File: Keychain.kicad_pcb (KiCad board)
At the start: 4 copper layers, 106.7 x 78.7 mm, 57 parts, among them J1 Micro_SD_Card, J2 Conn_01x04, U1 IMX6UL_BGA289, U2 DDR3_BGA96, U3 AZ1117C-3.3, U4 AZ1117C-1.5

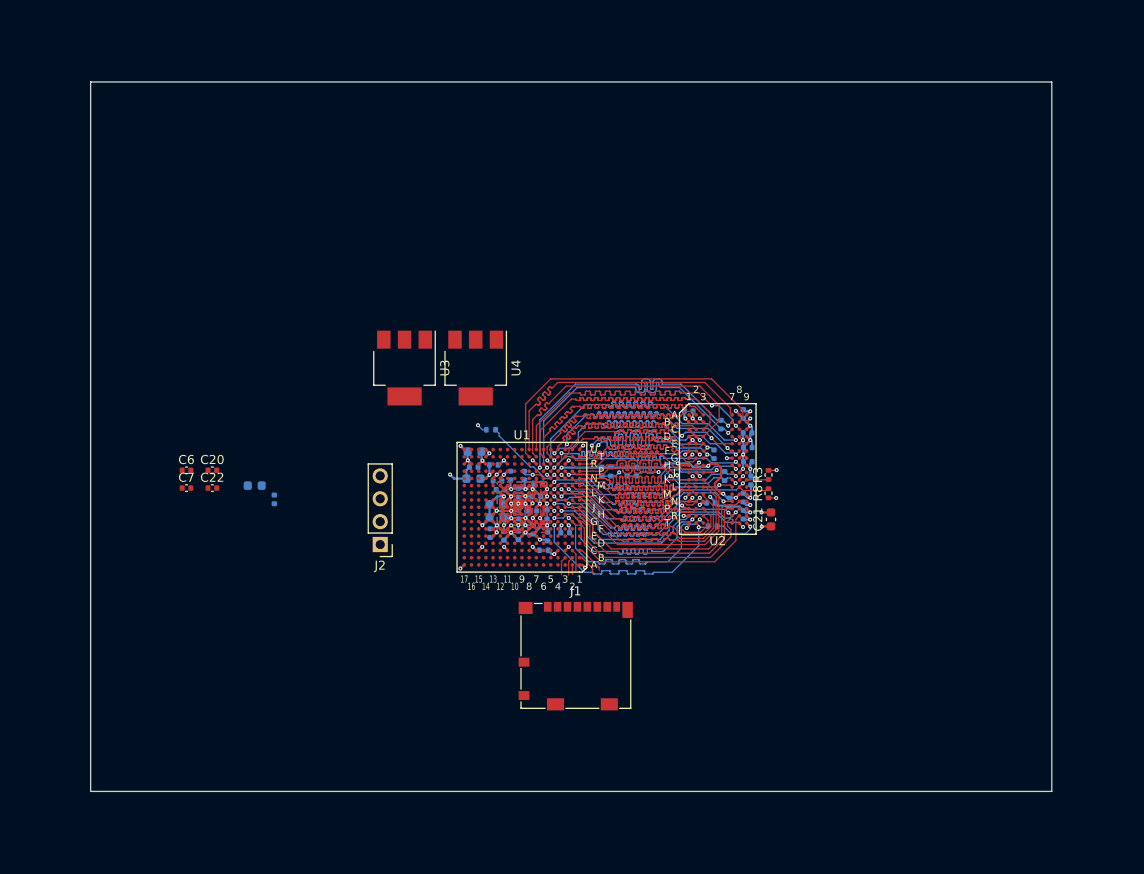
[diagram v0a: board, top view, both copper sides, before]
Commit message: Finished first version of board
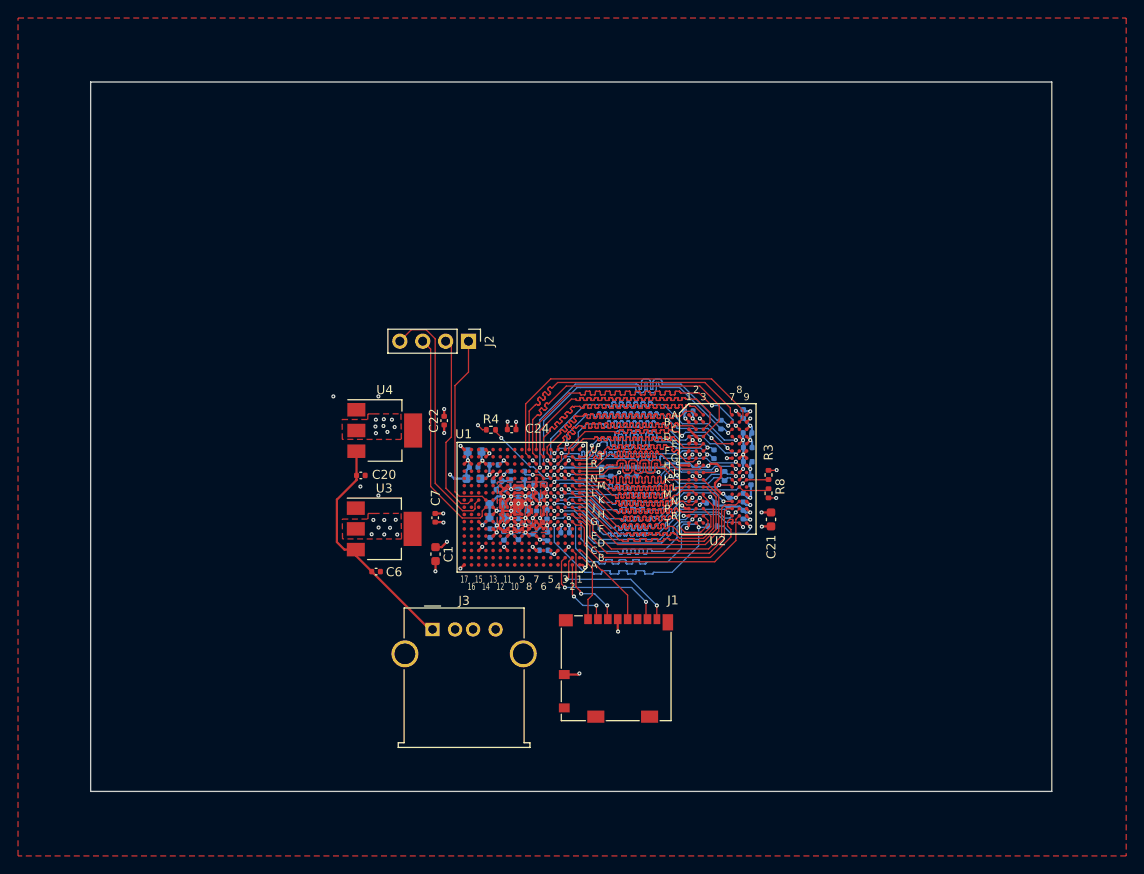
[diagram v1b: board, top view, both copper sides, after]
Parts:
- added J3: USB_A, Connector_USB:USB_A_Molex_67643_Horizontal, F.Cu at (137.0, 98.9)
- C1, C24, R4: moved to F.Cu
- moved C26 30.3 mm to (149.7, 86.1)
- moved C7 27.8 mm to (137.3, 86.5), turned to 90 degrees
- moved C22 26.8 mm to (138.3, 75.7), turned to 90 degrees
- moved J2 24.6 mm to (141.0, 66.9), turned to 270 degrees
- moved C6 23.9 mm to (130.7, 92.4)
- moved C1 21.5 mm to (137.3, 90.5), turned to 270 degrees
- moved U3 18.0 mm to (131.6, 87.7), turned to 0 degrees
- moved C20 16.5 mm to (129.1, 81.8)
- moved U4 12.2 mm to (131.7, 76.8), turned to 0 degrees
- moved C24 10.2 mm to (145.8, 76.7), turned to 180 degrees
- moved J1 4.68 mm to (157.4, 103.2)
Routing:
- net Debug_CTS: track 0.00 -> 27.8 mm
- net +5V: track 0.00 -> 26.0 mm
- net Debug_RTS: track 0.00 -> 24.9 mm
- net Debug_TX: track 0.00 -> 21.2 mm
- net Debug_RX: track 0.00 -> 20.5 mm
- net SD_D1: track 2.09 -> 15.4 mm, vias 0 -> 2
- net SD_D0: track 2.05 -> 15.3 mm, vias 0 -> 2
- net GND: track 111.4 -> 119.1 mm, vias 55 -> 64
- net SD_CMD: track 2.48 -> 10.2 mm, vias 0 -> 2
- net SD_D3: track 1.07 -> 8.07 mm, vias 0 -> 2
- net SD_CLK: track 3.26 -> 10.0 mm
- net SD_D2: track 2.40 -> 7.77 mm
- net +3V3: track 25.7 -> 29.6 mm, vias 9 -> 20
- net +1V5: track 34.9 -> 36.6 mm, vias 23 -> 33
- net /DDR/ZQPAD: vias 1 -> 2
